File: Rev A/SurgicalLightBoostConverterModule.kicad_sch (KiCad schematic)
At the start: 65 parts, among them Q1 IRLZ44N, Q2 IRLZ44N, Q3 BC337, Q4 BC327, Q5 BC327, U1 TL494, U2 TL431D, U3 LM358

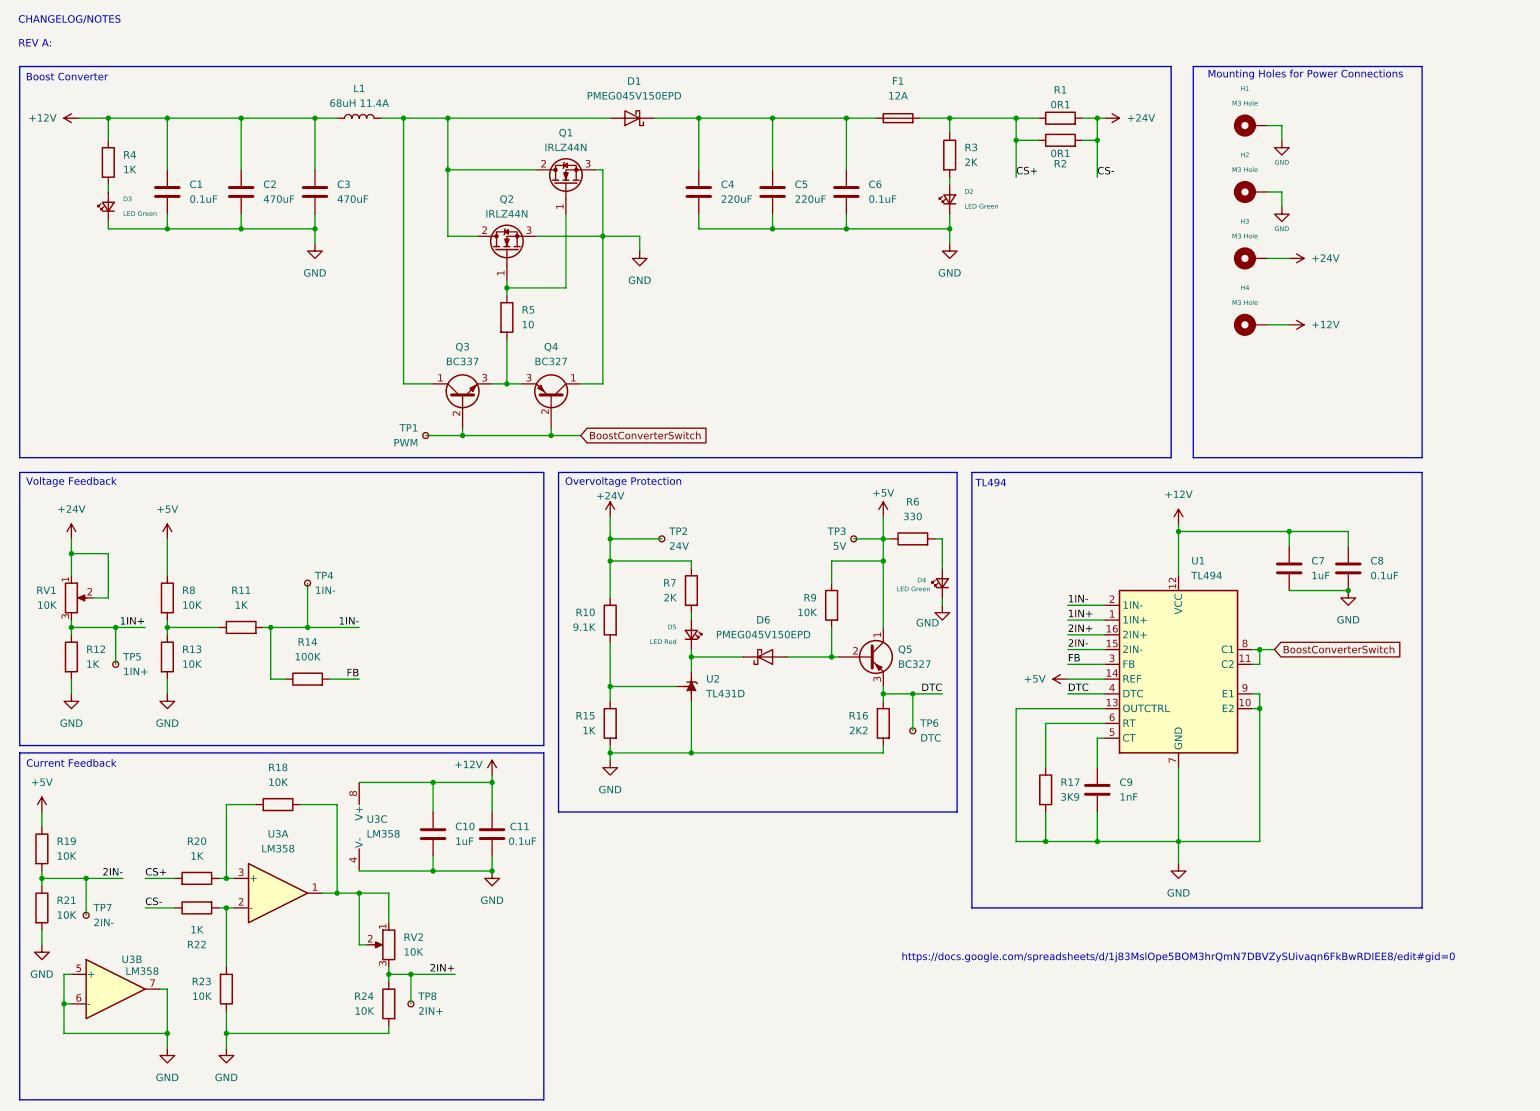
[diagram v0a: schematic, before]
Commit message: added michael's changes
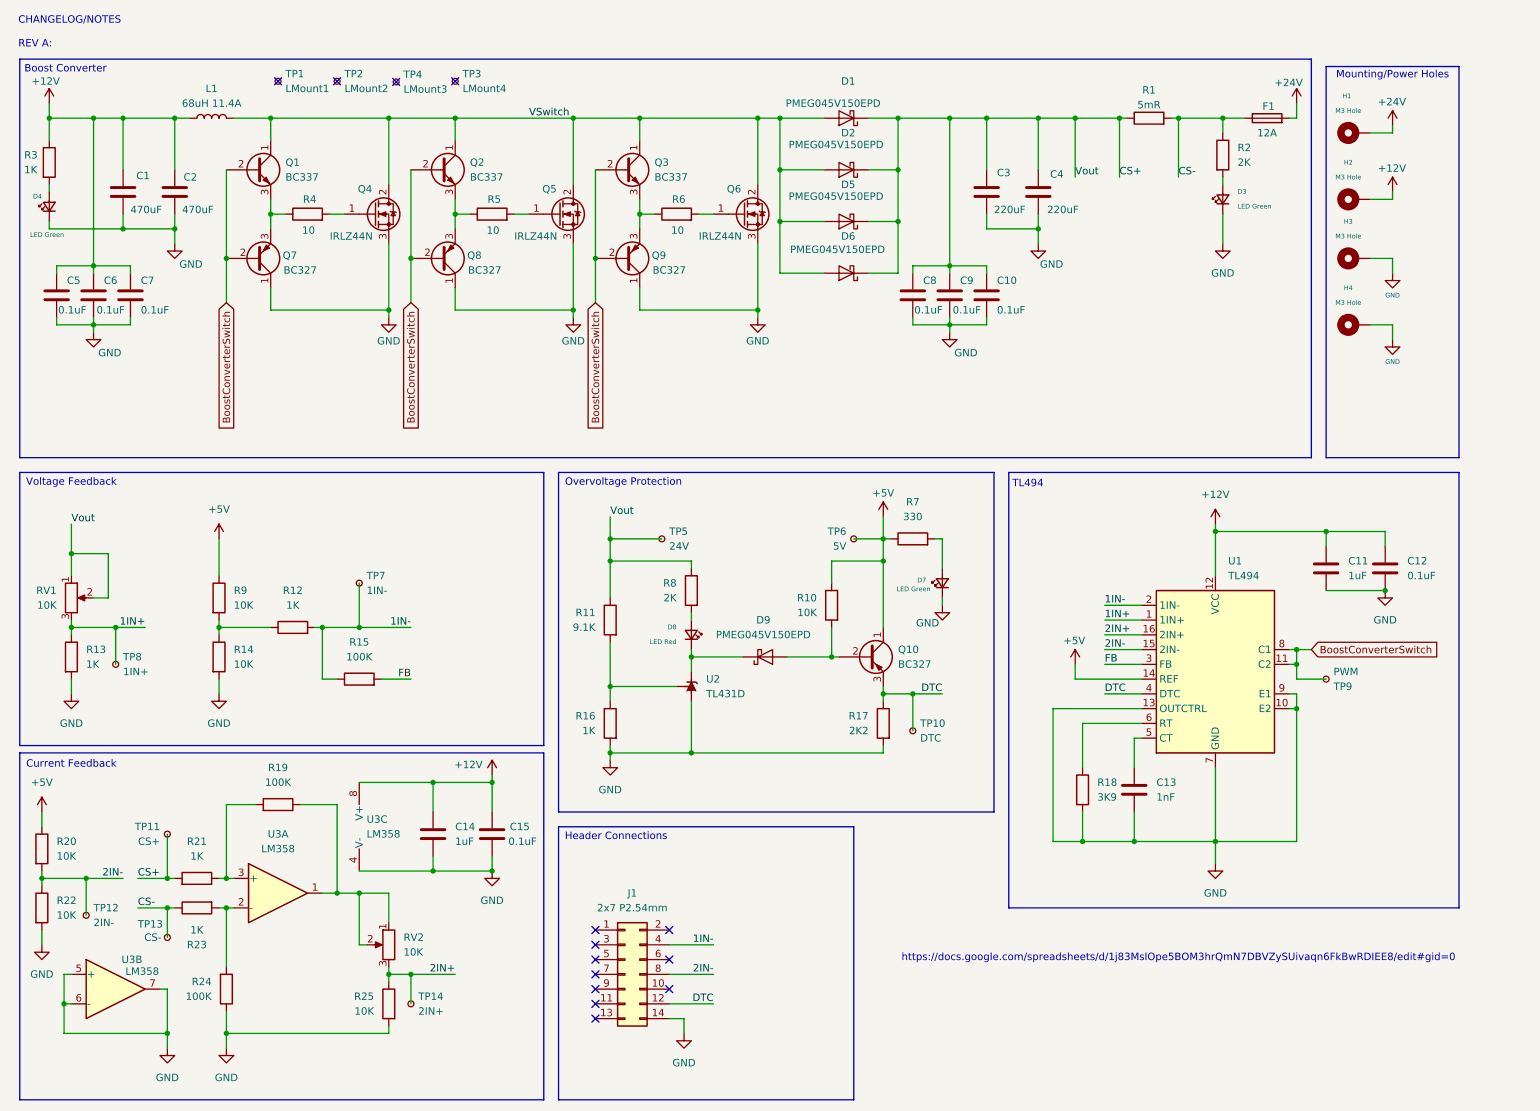
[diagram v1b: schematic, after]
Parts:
- removed Q1, Q2: IRLZ44N, Package_TO_SOT_THT:TO-220-3_Vertical, symbol Transistor_FET:IRLZ44N
- removed Q4: BC327, Package_TO_SOT_THT:TO-92_Inline, symbol Transistor_BJT:BC327
- removed R2: 0R1, Resistor_SMD:R_2512_6332Metric, symbol Device:R
- added C10, C7, C8, C9: 0.1uF, Capacitor_SMD:C_0805_2012Metric, symbol Device:C
- added D2, D5, D6: PMEG045V150EPD, Package_TO_SOT_SMD:Nexperia_CFP15_SOT-1289, symbol Diode:PMEG045V150EPD
- added J1: 2x7 P2.54mm, Connector_PinHeader_2.54mm:PinHeader_2x07_P2.54mm_Vertical, symbol Connector_Generic:Conn_02x07_Odd_Even
- added Q1, Q2: BC337, Package_TO_SOT_THT:TO-92_Inline, symbol Transistor_BJT:BC337
- added Q4, Q5, Q6: IRLZ44N, Package_TO_SOT_THT:TO-220-3_Vertical, symbol Transistor_FET:IRLZ44N
- added Q7, Q8, Q9: BC327, Package_TO_SOT_THT:TO-92_Inline, symbol Transistor_BJT:BC327
- added R4, R6: 10, Resistor_SMD:R_0805_2012Metric, symbol Device:R
- added TP11: CS+, TestPoint:TestPoint_Loop_D2.54mm_Drill1.5mm_Beaded, symbol Connector:TestPoint_Small
- added TP13: CS-, TestPoint:TestPoint_Loop_D2.54mm_Drill1.5mm_Beaded, symbol Connector:TestPoint_Small
- added TP2: LMount2, TestPoint:TestPoint_Loop_D2.54mm_Drill1.5mm_Beaded, symbol Connector:TestPoint_Small
- added TP3: LMount4, TestPoint:TestPoint_Loop_D2.54mm_Drill1.5mm_Beaded, symbol Connector:TestPoint_Small
- added TP4: LMount3, TestPoint:TestPoint_Loop_D2.54mm_Drill1.5mm_Beaded, symbol Connector:TestPoint_Small
- added TP9: PWM, TestPoint:TestPoint_Loop_D2.54mm_Drill1.5mm_Beaded, symbol Connector:TestPoint_Small
- F1: footprint Fuse:Fuse_1206_3216Metric_Pad1.42x1.75mm_HandSolder -> Fuse:Fuseholder_Clip-6.3x32mm_Littelfuse_102071_Inline_P34.70x7.60mm_D2.00mm_Horizontal
- R1: value 0R1 -> 5mR
- R19: renamed from R18; value 10K -> 100K
- R24: renamed from R23; value 10K -> 100K
- TP1: value PWM -> LMount1; footprint TestPoint:TestPoint_Pad_D2.0mm -> TestPoint:TestPoint_Loop_D2.54mm_Drill1.5mm_Beaded
- TP10: renamed from TP6; footprint TestPoint:TestPoint_Pad_D2.0mm -> TestPoint:TestPoint_Loop_D2.54mm_Drill1.5mm_Beaded
- TP12: renamed from TP7; footprint TestPoint:TestPoint_Pad_D2.0mm -> TestPoint:TestPoint_Loop_D2.54mm_Drill1.5mm_Beaded
- TP14: renamed from TP8; footprint TestPoint:TestPoint_Pad_D2.0mm -> TestPoint:TestPoint_Loop_D2.54mm_Drill1.5mm_Beaded
- TP5: renamed from TP2; footprint TestPoint:TestPoint_Pad_D2.0mm -> TestPoint:TestPoint_Loop_D2.54mm_Drill1.5mm_Beaded
- TP6: renamed from TP3; footprint TestPoint:TestPoint_Pad_D2.0mm -> TestPoint:TestPoint_Loop_D2.54mm_Drill1.5mm_Beaded
- TP7: renamed from TP4; footprint TestPoint:TestPoint_Pad_D2.0mm -> TestPoint:TestPoint_Loop_D2.54mm_Drill1.5mm_Beaded
- TP8: renamed from TP5; footprint TestPoint:TestPoint_Pad_D2.0mm -> TestPoint:TestPoint_Loop_D2.54mm_Drill1.5mm_Beaded
- U2: footprint Package_SO:SOIC-8_3.9x4.9mm_P1.27mm -> Package_DIP:DIP-8_W7.62mm_Socket
- renumbered C2 to C1, C7 to C11, C8 to C12, C9 to C13, C10 to C14, C11 to C15, C3 to C2, C4 to C3, C5 to C4, C1 to C5, D2 to D3, D3 to D4, D4 to D7, D5 to D8, D6 to D9, H3 to H1, H4 to H2, H1 to H3, H2 to H4, Q5 to Q10, R9 to R10, R10 to R11, R11 to R12, R12 to R13, R13 to R14, R14 to R15, R15 to R16, R16 to R17, R17 to R18, R3 to R2, R19 to R20, R20 to R21, R21 to R22, R22 to R23, R24 to R25, R4 to R3, R6 to R7, R7 to R8, R8 to R9
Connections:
- net +12V: now also C6.1, C7.1
- net +24V: now also F1.2; no longer R1.2, R11.1, R23.1, R8.1, RV1.1, RV1.2, TP5.1
- net 1IN-: now also J1.4 (Pin_4)
- net 2IN-: now also J1.8 (Pin_8)
- net BoostConverterSwitch: now also Q1.2 (B), Q2.2 (B), Q7.2 (B), Q8.2 (B), Q9.2 (B), TP9.1; no longer TP1.1
- net CS+: now also C3.1, C4.1, D1.3 (K), R11.1, R8.1, RV1.1, RV1.2, TP5.1, C10.1, C8.1, C9.1, D2.3 (K), D5.3 (K), D6.3 (K), TP11.1; no longer F1.2, R2.1
- net DTC: now also J1.12 (Pin_12)
- net GND: now also C10.2, C7.2, C8.2, C9.2, J1.14 (Pin_14), Q4.3 (S), Q5.3 (S), Q6.3 (S), Q7.1 (C), Q8.1 (C), Q9.1 (C)
- net VSwitch: now reaches D1.1 (A), D1.2 (A), L1.2, Q3.1 (C)
- net VSwitch: now also D2.1 (A), D2.2 (A), D5.1 (A), D5.2 (A), D6.1 (A), D6.2 (A), Q1.1 (C), Q2.1 (C), Q4.2 (D), Q5.2 (D), Q6.2 (D)
- net at Q3.3 (E): now also Q9.3 (E), R6.1; no longer R5.2
- net at R5.1: now also Q2.3 (E), Q8.3 (E)
- new net: Q1.3 (E), Q7.3 (E), R4.1
- new net: Q4.1 (G), R4.2
- new net: Q6.1 (G), R6.2
- new net: Q5.1 (G), R5.2
- new net CS-: F1.1, R1.2, R2.1, R23.1, TP13.1
- no-connect marks 0 -> 14
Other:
- note added: "Header Connections"
- note added: "Mounting/Power Holes"
- note removed: "Mounting Holes for Power Connections"
- moved on the sheet: C1, C11, C12, C13, C2, C3, C4, C5, D1, D3, D4, H1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
